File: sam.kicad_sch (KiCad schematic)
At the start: 57 parts, among them IC1 HYB4116, IC15 MC6883, IC16 74LS244N, IC2 HYB4116, IC3 HYB4116, IC31 74LS02N, IC33 74LS138N, IC4 HYB4116, IC5 HYB4116, IC6 HYB4116, IC7 HYB4116, IC8 HYB4116

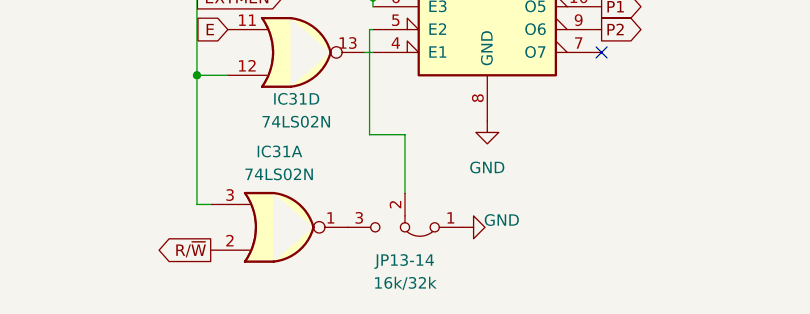
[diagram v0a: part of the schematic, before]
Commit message: refresh pcb
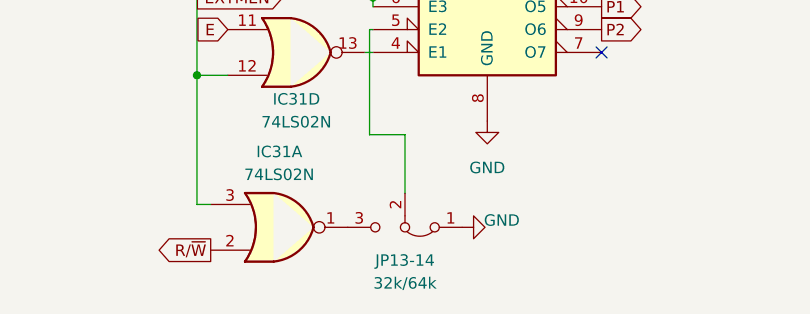
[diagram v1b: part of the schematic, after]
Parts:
- IC1, IC15, IC16, IC2, IC3, IC31, IC33, IC4, IC5, IC6, IC7, IC8: SA2120 (none) -> Sheet 1
- IC31: SA2120 (none) -> Sheet 1 (spare)
- JP13-14: value 16k/32k -> 32k/64k
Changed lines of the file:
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@@
+      (effects (font (size 1.27 1.27)) hide)
+    )
+    (property "SA2120" "Sheet 1" (id 5) (at 35.433 42.418 0)
       (effects (font (size 1.27 1.27)) hide)
     )
@@
     (in_bom yes) (on_board yes) (fields_autoplaced)
     (property "Reference" "JP13-14" (id 0) (at 112.903 199.39 0))
-    (property "Value" "16k/32k" (id 1) (at 112.903 201.93 0))
+    (property "Value" "32k/64k" (id 1) (at 112.903 201.93 0))
     (property "Footprint" "Connector_PinHeader_2.54mm:PinHeader_1x03_P2.54mm_Vertical" (id 2) (at 112.903 195.707 0)
       (effects (font (size 1.27 1.27)) hide)
@@
     )
     (property "Note" "use general 4164 with suitable timing" (id 4) (at 120.777 42.545 0)
+      (effects (font (size 1.27 1.27)) hide)
+    )
+    (property "SA2120" "Sheet 1" (id 5) (at 120.777 42.545 0)
       (effects (font (size 1.27 1.27)) hide)
     )
@@
     )
     (property "DigiKey" "296-1653-5-ND" (id 4) (at 35.306 168.91 0)
+      (effects (font (size 1.27 1.27)) hide)
+    )
+    (property "SA2120" "Sheet 1" (id 5) (at 35.306 168.91 0)
       (effects (font (size 1.27 1.27)) hide)
     )
@@
       (effects (font (size 1.27 1.27)) hide)
     )
+    (property "SA2120" "Sheet 1" (id 5) (at 100.838 176.276 0)
+      (effects (font (size 1.27 1.27)) hide)
+    )
     (pin "11")
     (pin "12")
@@
     )
     (property "DigiKey" "296-1639-5-ND" (id 4) (at 122.047 166.116 0)
+      (effects (font (size 1.27 1.27)) hide)
+    )
+    (property "SA2120" "Sheet 1" (id 5) (at 122.047 166.116 0)
       (effects (font (size 1.27 1.27)) hide)
     )
@@
       (effects (font (size 1.27 1.27)) hide)
     )
+    (property "SA2120" "Sheet 1" (id 5) (at 78.105 42.418 0)
+      (effects (font (size 1.27 1.27)) hide)
+    )
     (pin "1")
     (pin "10")
@@
       (effects (font (size 1.27 1.27)) hide)
     )
+    (property "SA2120" "Sheet 1" (id 5) (at 236.22 124.333 0)
+      (effects (font (size 1.27 1.27)) hide)
+    )
     (pin "4")
     (pin "5")
@@
       (effects (font (size 1.27 1.27)) hide)
     )
+    (property "SA2120" "Sheet 1 (spare)" (id 5) (at 98.933 195.707 0)
+      (effects (font (size 1.27 1.27)) hide)
+    )
     (pin "1")
     (pin "2")
@@
     )
     (property "Note" "use general 4164 with suitable timing" (id 4) (at 120.777 103.251 0)
+      (effects (font (size 1.27 1.27)) hide)
+    )
+    (property "SA2120" "Sheet 1" (id 5) (at 120.777 103.251 0)
       (effects (font (size 1.27 1.27)) hide)
     )
@@
       (effects (font (size 1.27 1.27)) hide)
     )
+    (property "SA2120" "Sheet 1" (id 5) (at 35.433 103.124 0)
+      (effects (font (size 1.27 1.27)) hide)
+    )
     (pin "1")
     (pin "10")
@@
       (effects (font (size 1.27 1.27)) hide)
     )
+    (property "SA2120" "Sheet 1" (id 5) (at 163.449 103.251 0)
+      (effects (font (size 1.27 1.27)) hide)
+    )
     (pin "1")
     (pin "10")
@@
       (effects (font (size 1.27 1.27)) hide)
     )
+    (property "SA2120" "Sheet 1" (id 5) (at 163.449 42.545 0)
+      (effects (font (size 1.27 1.27)) hide)
+    )
     (pin "1")
     (pin "10")
@@
       (effects (font (size 1.27 1.27)) hide)
     )
+    (property "SA2120" "Sheet 1" (id 5) (at 78.105 103.124 0)
+      (effects (font (size 1.27 1.27)) hide)
+    )
     (pin "1")
     (pin "10")
@@
       (effects (font (size 1.27 1.27)) hide)
     )
+    (property "SA2120" "Sheet 1" (id 6) (at 244.856 60.071 0)
+      (effects (font (size 1.27 1.27)) hide)
+    )
